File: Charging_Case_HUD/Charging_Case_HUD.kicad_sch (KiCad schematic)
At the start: 31 parts, among them J1 Conn_01x20, J2 09551296822741, J3 Conn_01x02, J4 Conn_01x02, J5 Conn_01x02, SW1 SW_MEC_5G, SW2 SW_DIP_x01, U1 ILI9163C

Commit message: with layout
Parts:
- J1: footprint Connector_PinHeader_2.54mm:PinHeader_1x20_P2.54mm_Vertical -> Connector_Molex:Molex_Micro-Fit_3.0_43045-2010_2x10-1MP_P3.00mm_Horizontal
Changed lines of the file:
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@@
     (property "Reference" "J1" (id 0) (at 13.335 39.37 90))
     (property "Value" "Conn_01x20" (id 1) (at 15.875 39.37 90))
-    (property "Footprint" "Connector_PinHeader_2.54mm:PinHeader_1x20_P2.54mm_Vertical" (id 2) (at 19.685 39.37 0)
+    (property "Footprint" "Connector_Molex:Molex_Micro-Fit_3.0_43045-2010_2x10-1MP_P3.00mm_Horizontal" (id 2) (at 19.685 39.37 0)
       (effects (font (size 1.27 1.27)) hide)
     )
@@
     )
     (path "/47d61bda-e1d0-4382-b01d-06c237dc658e"
-      (reference "J1") (unit 1) (value "Conn_01x20") (footprint "Connector_PinHeader_2.54mm:PinHeader_1x20_P2.54mm_Vertical")
+      (reference "J1") (unit 1) (value "Conn_01x20") (footprint "Connector_Molex:Molex_Micro-Fit_3.0_43045-2010_2x10-1MP_P3.00mm_Horizontal")
     )
     (path "/253d4602-5d1f-477f-8c18-29c7efc6e641"

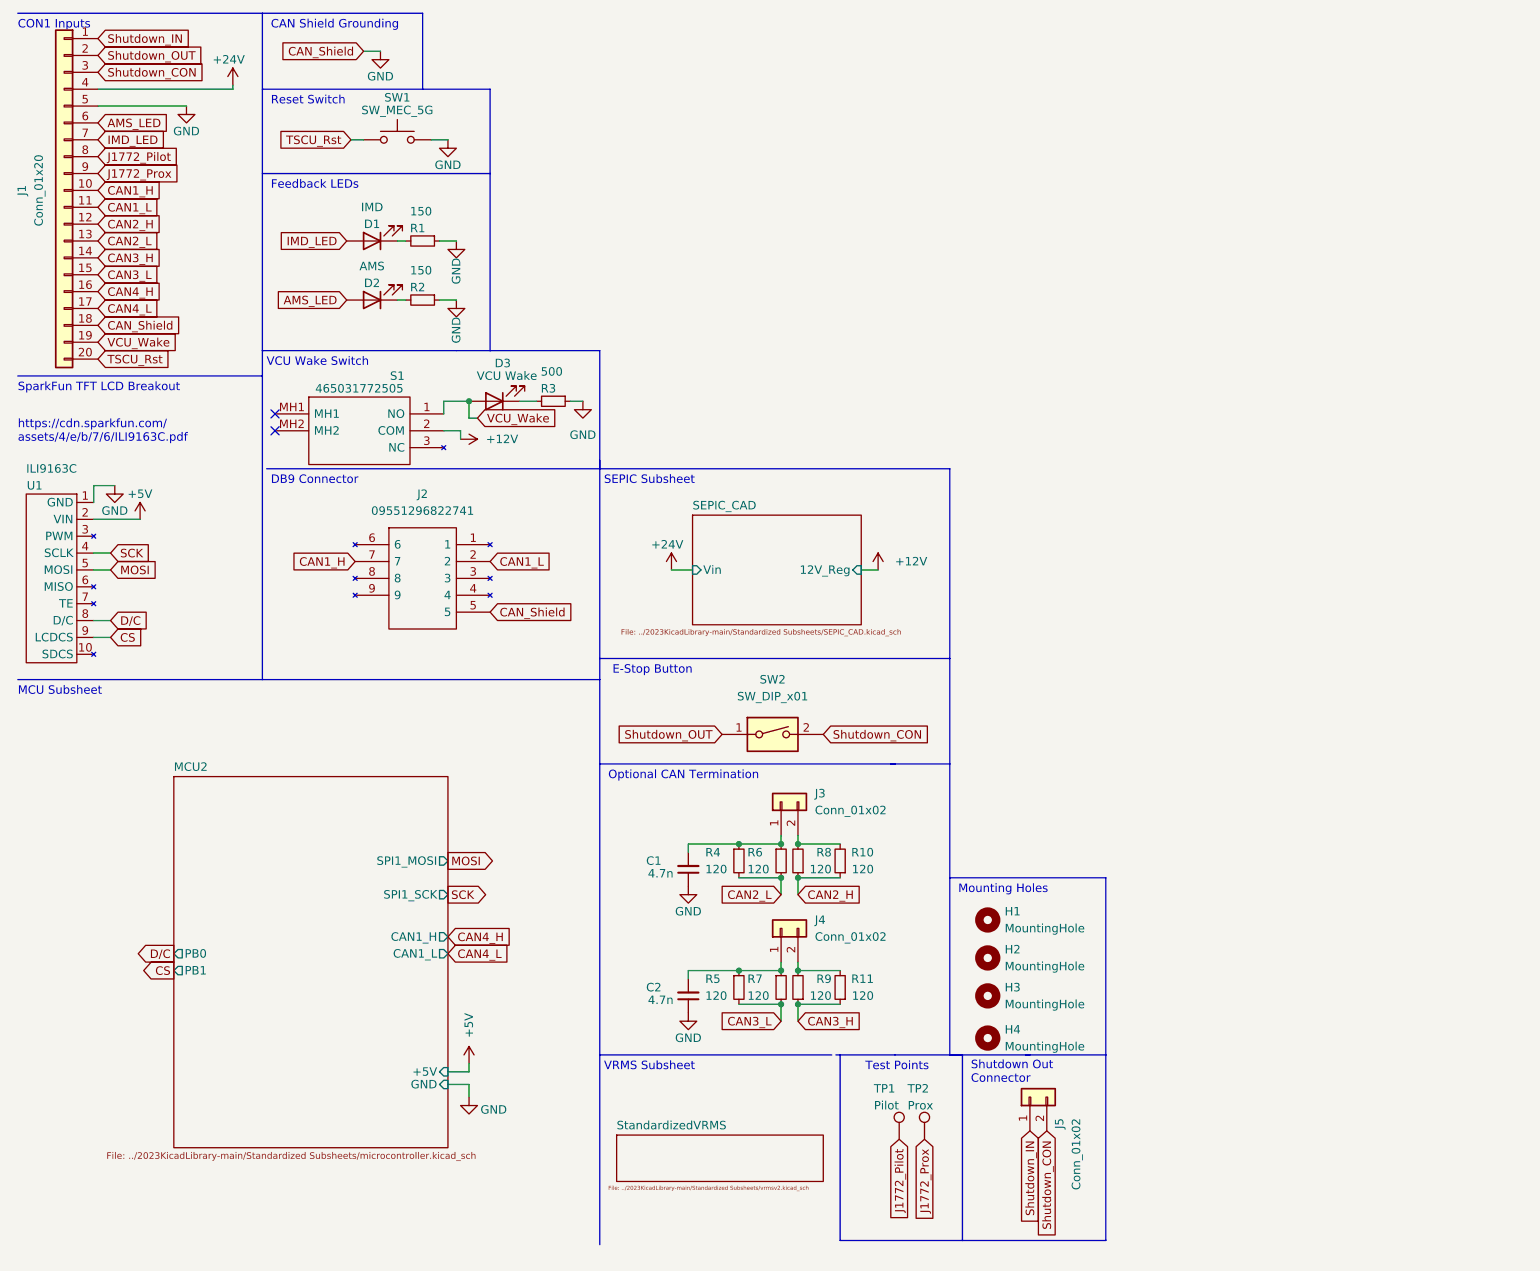
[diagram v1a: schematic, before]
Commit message: new HUD PCB
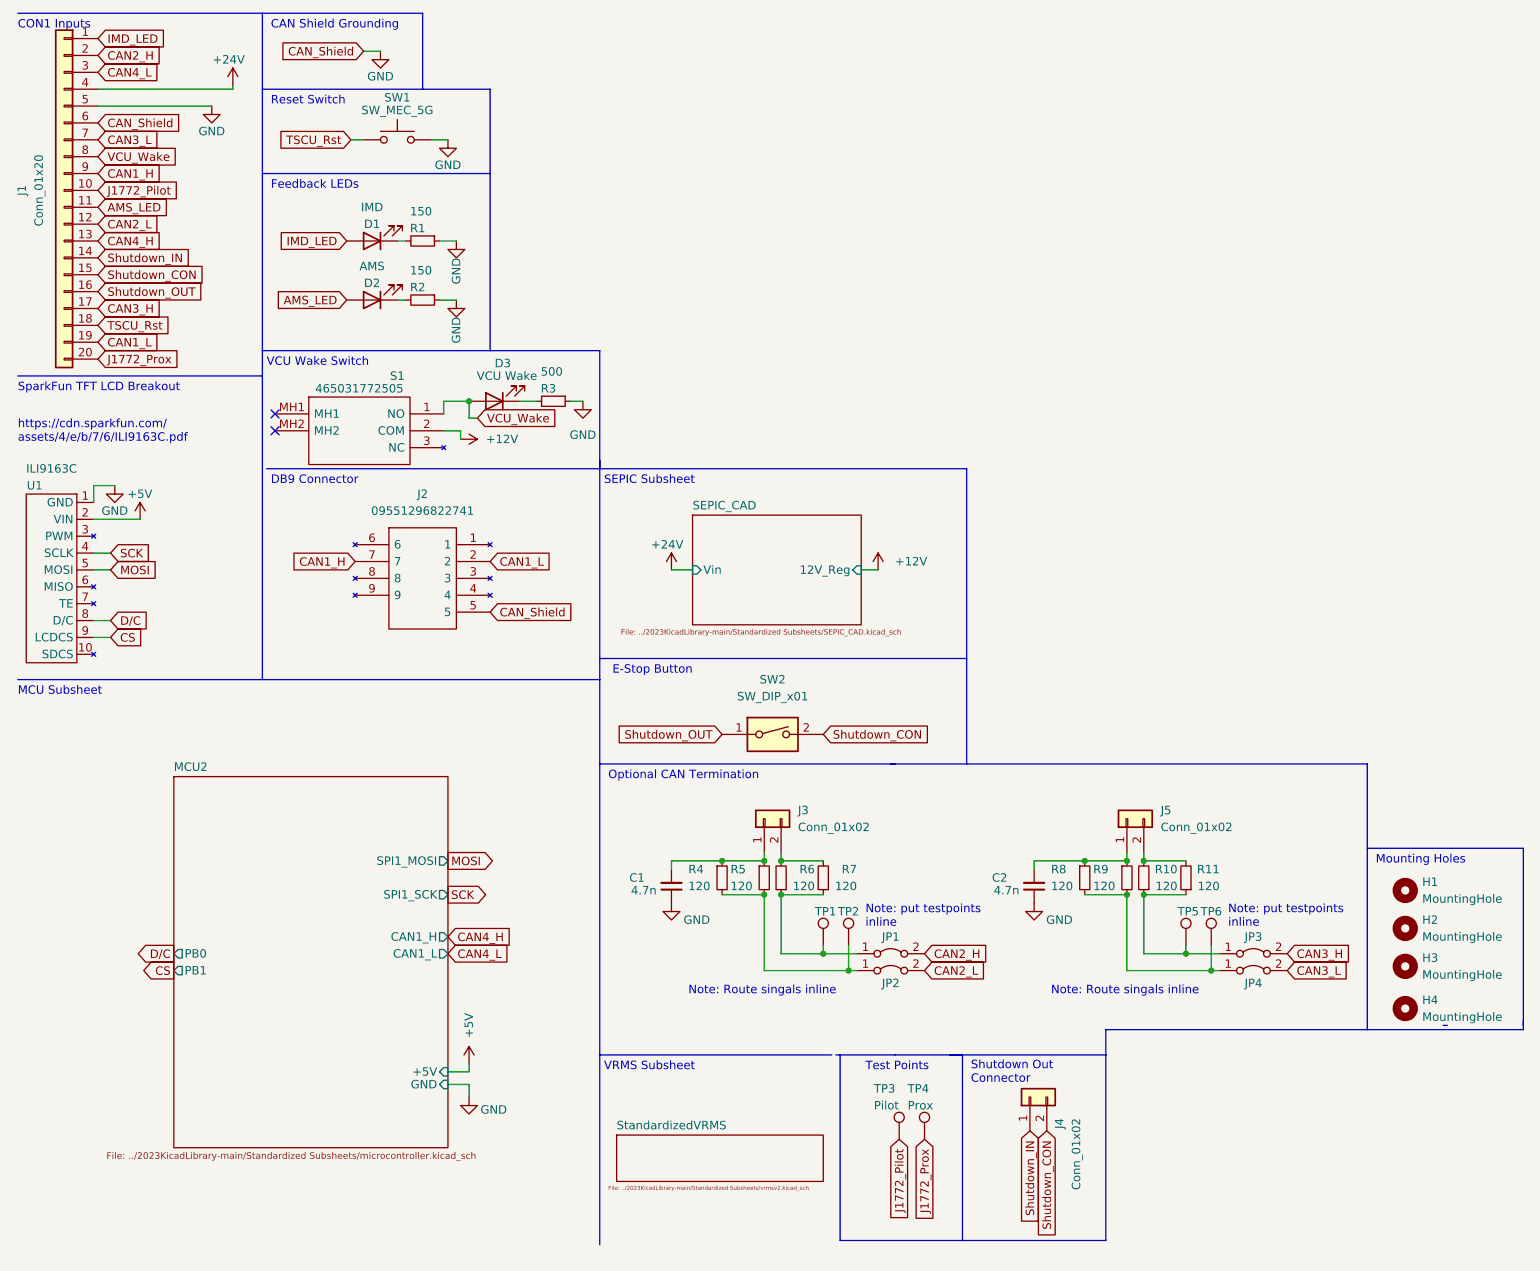
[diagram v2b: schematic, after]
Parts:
- removed J4: Conn_01x02, Connector_PinHeader_2.54mm:PinHeader_1x02_P2.54mm_Vertical, symbol Connector_Generic:Conn_01x02
- added J5: Conn_01x02, Connector_PinHeader_2.54mm:PinHeader_1x02_P2.54mm_Vertical, symbol Connector_Generic:Conn_01x02
- added JP1, JP2, JP3, JP4: (no value), Jumper:SolderJumper-2_P1.3mm_Bridged2Bar_Pad1.0x1.5mm, symbol Jumper:Jumper_2_Bridged
- added TP1, TP2, TP5, TP6: (no value), TestPoint:TestPoint_THTPad_1.0x1.0mm_Drill0.5mm, symbol Connector:TestPoint
- D2: footprint LED_SMD:LED_0805_2012Metric -> LED_SMD:LED_0603_1608Metric
- SW2: footprint Connector:Banana_Jack_2Pin -> Connector_Wire:SolderWire-0.1sqmm_1x02_P3.6mm_D0.4mm_OD1mm
- renumbered J5 to J4, TP1 to TP3, TP2 to TP4
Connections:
- net AMS_LED: now also J1.11 (Pin_11); no longer J1.6 (Pin_6)
- net CAN1_H: now also J1.9 (Pin_9); no longer J1.10 (Pin_10)
- net CAN1_L: now also J1.19 (Pin_19); no longer J1.11 (Pin_11)
- net CAN2_H: now also J1.2 (Pin_2), JP1.2 (B); no longer J1.12 (Pin_12), R10.1, R8.1
- net CAN2_L: now also J1.12 (Pin_12), JP2.2 (B); no longer J1.13 (Pin_13), R4.2, R6.2
- net CAN3_H: now also J1.17 (Pin_17), JP3.2 (B); no longer J1.14 (Pin_14), R11.1, R9.1
- net CAN3_L: now also J1.7 (Pin_7), JP4.2 (B); no longer J1.15 (Pin_15), R5.2, R7.2
- net CAN4_H: now also J1.13 (Pin_13); no longer J1.16 (Pin_16)
- net CAN4_L: now also J1.3 (Pin_3); no longer J1.17 (Pin_17)
- net GND: now also J1.6 (Pin_6); no longer J1.18 (Pin_18)
- net IMD_LED: now also J1.1 (Pin_1); no longer J1.7 (Pin_7)
- net J1772_Pilot: now also J1.10 (Pin_10); no longer J1.8 (Pin_8)
- net J1772_Prox: now also J1.20 (Pin_20); no longer J1.9 (Pin_9)
- net Shutdown_CON: now also J1.15 (Pin_15); no longer J1.3 (Pin_3)
- net Shutdown_IN: now also J1.14 (Pin_14); no longer J1.1 (Pin_1)
- net Shutdown_OUT: now also J1.16 (Pin_16); no longer J1.2 (Pin_2)
- net TSCU_Rst: now also J1.18 (Pin_18); no longer J1.20 (Pin_20)
- net VCU_Wake: now also J1.8 (Pin_8); no longer J1.19 (Pin_19)
- net at C1.2, J3.1 (Pin_1), R4.1: now also R5.1; no longer R6.1
- net at R9.2: now also R8.2, JP4.1 (A), TP6.1; no longer R11.2
- new net: C2.2, J5.1 (Pin_1), R8.1, R9.1
- new net: JP2.1 (A), R4.2, R5.2, TP2.1
- new net: JP1.1 (A), R6.1, R7.1, TP1.1
- new net: J3.2 (Pin_2), R6.2, R7.2
- new net: J5.2 (Pin_2), R10.2, R11.2
- new net: JP3.1 (A), R10.1, R11.1, TP5.1
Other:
- note added: "Note: Route singals inline"
- note added: "Note: put testpoints inline"
